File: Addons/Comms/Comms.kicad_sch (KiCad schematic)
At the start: 12 parts, among them J1 Conn_01x02, J2 Conn_02x06_Odd_Even, J3 Conn_01x02, J4 Conn_01x01, U1 SP3485EN

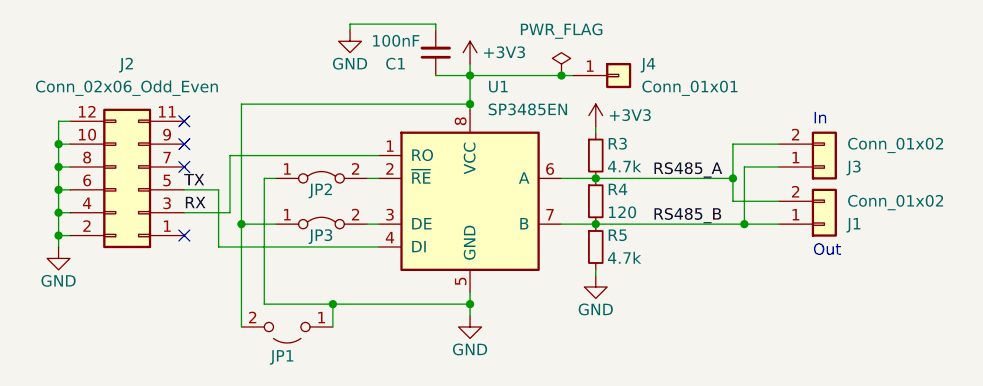
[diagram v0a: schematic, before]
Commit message: don't bridge 3v3 and ground lol
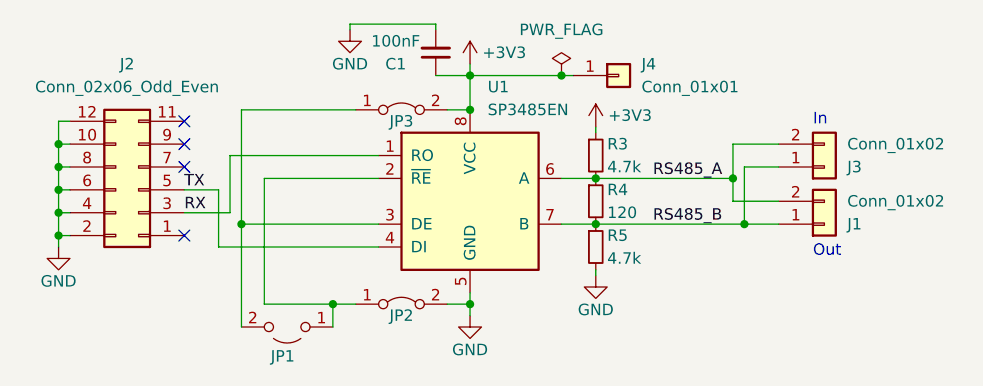
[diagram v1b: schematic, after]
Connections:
- net +3V3: now also JP3.2 (B); no longer JP1.2 (B), JP3.1 (A)
- net GND: now also JP2.2 (B); no longer JP1.1 (A), JP2.1 (A)
- net at U1.2 (~{RE}): now also JP1.1 (A), JP2.1 (A); no longer JP2.2 (B)
- net at U1.3 (DE): now also JP1.2 (B), JP3.1 (A); no longer JP3.2 (B)
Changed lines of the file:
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@@
   (junction (at 176.53 93.98) (diameter 0) (color 0 0 0 0)
   )
+  (junction (at 162.56 81.28) (diameter 0) (color 0 0 0 0)
+  )
   (junction (at 116.84 87.63) (diameter 0) (color 0 0 0 0)
   )
@@
   )
   (junction (at 116.84 90.17) (diameter 0) (color 0 0 0 0)
-  )
-  (junction (at 162.56 80.645) (diameter 0) (color 0 0 0 0)
   )
   (junction (at 116.84 92.71) (diameter 0) (color 0 0 0 0)
@@
     (stroke (width 0) (type default))
   )
-  (wire (pts (xy 147.32 102.87) (xy 162.56 102.87))
+  (wire (pts (xy 147.32 102.87) (xy 149.86 102.87))
     (stroke (width 0) (type default))
   )
@@
     (stroke (width 0) (type default))
   )
-  (wire (pts (xy 151.13 93.98) (xy 152.4 93.98))
-    (stroke (width 0) (type default))
-  )
   (wire (pts (xy 116.84 85.09) (xy 116.84 87.63))
     (stroke (width 0) (type default))
@@
     (stroke (width 0) (type default))
   )
+  (wire (pts (xy 160.02 102.87) (xy 162.56 102.87))
+    (stroke (width 0) (type default))
+  )
   (wire (pts (xy 130.81 90.17) (xy 134.62 90.17))
     (stroke (width 0) (type default))
@@
     (stroke (width 0) (type default))
   )
+  (wire (pts (xy 162.56 77.47) (xy 162.56 81.28))
+    (stroke (width 0) (type default))
+  )
   (wire (pts (xy 134.62 90.17) (xy 134.62 96.52))
     (stroke (width 0) (type default))
@@
     (stroke (width 0) (type default))
   )
-  (wire (pts (xy 140.97 88.9) (xy 139.7 88.9))
-    (stroke (width 0) (type default))
-  )
   (wire (pts (xy 149.225 71.755) (xy 158.75 71.755))
     (stroke (width 0) (type default))
@@
     (stroke (width 0) (type default))
   )
-  (wire (pts (xy 137.16 80.645) (xy 162.56 80.645))
+  (wire (pts (xy 137.16 81.28) (xy 149.86 81.28))
     (stroke (width 0) (type default))
   )
@@
     (stroke (width 0) (type default))
   )
-  (wire (pts (xy 137.16 93.98) (xy 137.16 80.645))
+  (wire (pts (xy 137.16 93.98) (xy 137.16 81.28))
     (stroke (width 0) (type default))
   )
@@
     (stroke (width 0) (type default))
   )
+  (wire (pts (xy 160.02 81.28) (xy 162.56 81.28))
+    (stroke (width 0) (type default))
+  )
   (wire (pts (xy 116.84 87.63) (xy 118.11 87.63))
     (stroke (width 0) (type default))
@@
     (stroke (width 0) (type default))
   )
-  (wire (pts (xy 152.4 88.9) (xy 151.13 88.9))
+  (wire (pts (xy 139.7 88.9) (xy 152.4 88.9))
     (stroke (width 0) (type default))
   )
@@
     (stroke (width 0) (type default))
   )
-  (wire (pts (xy 162.56 80.645) (xy 162.56 81.28))
-    (stroke (width 0) (type default))
-  )
   (wire (pts (xy 116.84 92.71) (xy 116.84 95.25))
     (stroke (width 0) (type default))
   )
-  (wire (pts (xy 137.16 93.98) (xy 140.97 93.98))
+  (wire (pts (xy 137.16 93.98) (xy 152.4 93.98))
     (stroke (width 0) (type default))
   )
   (wire (pts (xy 162.56 76.2) (xy 162.56 77.47))
-    (stroke (width 0) (type default))
-  )
-  (wire (pts (xy 162.56 77.47) (xy 162.56 80.645))
     (stroke (width 0) (type default))
   )
@@
         (path "/825aa7ba-79cf-4288-9f62-f278431e5a92"
           (reference "J1") (unit 1)
-        )
-      )
-    )
-  )
-  (symbol (lib_id "Jumper:Jumper_2_Bridged") (at 146.05 88.9 0) (unit 1)
-    (in_bom yes) (on_board yes) (dnp no)
-    (property "Reference" "JP2" (at 146.05 90.17 0)
-      (effects (font (size 1.27 1.27)))
-    )
-    (property "Value" "Jumper_2_Bridged" (at 146.05 86.36 0)
-      (effects (font (size 1.27 1.27)) hide)
-    )
-    (property "Footprint" "Jumper:SolderJumper-2_P1.3mm_Bridged_RoundedPad1.0x1.5mm" (at 146.05 88.9 0)
-      (effects (font (size 1.27 1.27)) hide)
-    )
-    (property "Datasheet" "~" (at 146.05 88.9 0)
-      (effects (font (size 1.27 1.27)) hide)
-    )
-    (pin "1")
-    (pin "2")
-    (instances
-      (project "Comms"
-        (path "/825aa7ba-79cf-4288-9f62-f278431e5a92"
-          (reference "JP2") (unit 1)
         )
       )
@@
     )
   )
-  (symbol (lib_id "Jumper:Jumper_2_Bridged") (at 146.05 93.98 0) (unit 1)
-    (in_bom yes) (on_board yes) (dnp no)
-    (property "Reference" "JP3" (at 146.05 95.25 0)
-      (effects (font (size 1.27 1.27)))
-    )
-    (property "Value" "Jumper_2_Bridged" (at 146.05 91.44 0)
-      (effects (font (size 1.27 1.27)) hide)
-    )
-    (property "Footprint" "Jumper:SolderJumper-2_P1.3mm_Bridged_RoundedPad1.0x1.5mm" (at 146.05 93.98 0)
-      (effects (font (size 1.27 1.27)) hide)
-    )
-    (property "Datasheet" "~" (at 146.05 93.98 0)
-      (effects (font (size 1.27 1.27)) hide)
-    )
-    (pin "1")
-    (pin "2")
-    (instances
-      (project "Comms"
-        (path "/825aa7ba-79cf-4288-9f62-f278431e5a92"
-          (reference "JP3") (unit 1)
-        )
-      )
-    )
-  )
   (symbol (lib_id "Connector_Generic:Conn_01x02") (at 201.93 87.63 0) (mirror x) (unit 1)
     (in_bom yes) (on_board yes) (dnp no)
@@
     )
   )
+  (symbol (lib_id "Jumper:Jumper_2_Bridged") (at 154.94 102.87 0) (unit 1)
+    (in_bom yes) (on_board yes) (dnp no)
+    (property "Reference" "JP2" (at 154.94 104.14 0)
+      (effects (font (size 1.27 1.27)))
+    )
+    (property "Value" "Jumper_2_Bridged" (at 154.94 100.33 0)
+      (effects (font (size 1.27 1.27)) hide)
+    )
+    (property "Footprint" "Jumper:SolderJumper-2_P1.3mm_Bridged_RoundedPad1.0x1.5mm" (at 154.94 102.87 0)
+      (effects (font (size 1.27 1.27)) hide)
+    )
+    (property "Datasheet" "~" (at 154.94 102.87 0)
+      (effects (font (size 1.27 1.27)) hide)
+    )
+    (pin "1")
+    (pin "2")
+    (instances
+      (project "Comms"
+        (path "/825aa7ba-79cf-4288-9f62-f278431e5a92"
+          (reference "JP2") (unit 1)
+        )
+      )
+    )
+  )
   (symbol (lib_id "power:GND") (at 176.53 99.695 0) (unit 1)
     (in_bom yes) (on_board yes) (dnp no)
@@
         )
       )
+    )
+  )
+  (symbol (lib_id "Jumper:Jumper_2_Bridged") (at 154.94 81.28 0) (unit 1)
+    (in_bom yes) (on_board yes) (dnp no)
+    (property "Reference" "JP3" (at 154.94 82.55 0)
+      (effects (font (size 1.27 1.27)))
+    )
+    (property "Value" "Jumper_2_Bridged" (at 154.94 78.74 0)
+      (effects (font (size 1.27 1.27)) hide)
+    )
+    (property "Footprint" "Jumper:SolderJumper-2_P1.3mm_Bridged_RoundedPad1.0x1.5mm" (at 154.94 81.28 0)
+      (effects (font (size 1.27 1.27)) hide)
+    )
+    (property "Datasheet" "~" (at 154.94 81.28 0)
+      (effects (font (size 1.27 1.27)) hide)
+    )
+    (pin "1")
+    (pin "2")
+    (instances
+      (project "Comms"
+        (path "/825aa7ba-79cf-4288-9f62-f278431e5a92"
+          (reference "JP3") (unit 1)
+        )
+      )

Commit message: Add RS485 functionality & addons, several fixes
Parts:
- C1: LCSC (none) -> C49678
- J1, J3: footprint Connector_PinHeader_2.54mm:PinHeader_1x02_P2.54mm_Horizontal -> Connector_JST:JST_XH_S2B-XH-A_1x02_P2.50mm_Horizontal
- R3, R5: LCSC (none) -> C17673
- R4: LCSC (none) -> C17437
- U1: LCSC (none) -> C8963
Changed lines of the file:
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@@
     (effects (font (size 1.27 1.27)) (justify left bottom))
-  )
-  (symbol (lib_id "Connector_Generic:Conn_01x02") (at 201.93 93.98 0) (mirror x) (unit 1)
-    (in_bom yes) (on_board yes) (dnp no)
-    (property "Reference" "J1" (at 204.47 93.98 0)
-      (effects (font (size 1.27 1.27)) (justify left))
-    )
-    (property "Value" "Conn_01x02" (at 204.47 91.44 0)
-      (effects (font (size 1.27 1.27)) (justify left))
-    )
-    (property "Footprint" "Connector_PinHeader_2.54mm:PinHeader_1x02_P2.54mm_Horizontal" (at 201.93 93.98 0)
-      (effects (font (size 1.27 1.27)) hide)
-    )
-    (property "Datasheet" "~" (at 201.93 93.98 0)
-      (effects (font (size 1.27 1.27)) hide)
-    )
-    (pin "1")
-    (pin "2")
-    (instances
-      (project "Comms"
-        (path "/825aa7ba-79cf-4288-9f62-f278431e5a92"
-          (reference "J1") (unit 1)
-        )
-      )
-    )
   )
   (symbol (lib_id "power:+3V3") (at 162.56 76.2 0) (unit 1)
@@
     )
     (property "Datasheet" "~" (at 125.73 90.17 0)
+      (effects (font (size 1.27 1.27)) hide)
+    )
+    (property "LCSC" "" (at 125.73 90.17 0)
       (effects (font (size 1.27 1.27)) hide)
     )
@@
       (effects (font (size 1.27 1.27)) hide)
     )
+    (property "LCSC" "C17673" (at 176.53 96.52 0)
+      (effects (font (size 1.27 1.27)) hide)
+    )
     (pin "1")
     (pin "2")
@@
       (effects (font (size 1.27 1.27)) hide)
     )
+    (property "LCSC" "C17673" (at 176.53 86.36 0)
+      (effects (font (size 1.27 1.27)) hide)
+    )
     (pin "1")
     (pin "2")
@@
     )
   )
+  (symbol (lib_id "Connector_Generic:Conn_01x02") (at 201.93 87.63 0) (mirror x) (unit 1)
+    (in_bom yes) (on_board yes) (dnp no)
+    (property "Reference" "J3" (at 204.47 87.63 0)
+      (effects (font (size 1.27 1.27)) (justify left))
+    )
+    (property "Value" "Conn_01x02" (at 204.47 85.09 0)
+      (effects (font (size 1.27 1.27)) (justify left))
+    )
+    (property "Footprint" "Connector_JST:JST_XH_S2B-XH-A_1x02_P2.50mm_Horizontal" (at 201.93 87.63 0)
+      (effects (font (size 1.27 1.27)) hide)
+    )
+    (property "Datasheet" "~" (at 201.93 87.63 0)
+      (effects (font (size 1.27 1.27)) hide)
+    )
+    (property "LCSC" "" (at 201.93 87.63 0)
+      (effects (font (size 1.27 1.27)) hide)
+    )
+    (pin "1")
+    (pin "2")
+    (instances
+      (project "Comms"
+        (path "/825aa7ba-79cf-4288-9f62-f278431e5a92"
+          (reference "J3") (unit 1)
+        )
+      )
+    )
+  )
   (symbol (lib_id "power:GND") (at 149.225 72.39 0) (unit 1)
     (in_bom yes) (on_board yes) (dnp no)
@@
       (effects (font (size 1.27 1.27)) hide)
     )
+    (property "LCSC" "C49678" (at 158.75 74.93 0)
+      (effects (font (size 1.27 1.27)) hide)
+    )
     (pin "1")
     (pin "2")
@@
     )
   )
-  (symbol (lib_id "Connector_Generic:Conn_01x02") (at 201.93 87.63 0) (mirror x) (unit 1)
-    (in_bom yes) (on_board yes) (dnp no)
-    (property "Reference" "J3" (at 204.47 87.63 0)
-      (effects (font (size 1.27 1.27)) (justify left))
-    )
-    (property "Value" "Conn_01x02" (at 204.47 85.09 0)
-      (effects (font (size 1.27 1.27)) (justify left))
-    )
-    (property "Footprint" "Connector_PinHeader_2.54mm:PinHeader_1x02_P2.54mm_Horizontal" (at 201.93 87.63 0)
-      (effects (font (size 1.27 1.27)) hide)
-    )
-    (property "Datasheet" "~" (at 201.93 87.63 0)
-      (effects (font (size 1.27 1.27)) hide)
-    )
-    (pin "1")
-    (pin "2")
-    (instances
-      (project "Comms"
-        (path "/825aa7ba-79cf-4288-9f62-f278431e5a92"
-          (reference "J3") (unit 1)
+  (symbol (lib_id "Connector_Generic:Conn_01x02") (at 201.93 93.98 0) (mirror x) (unit 1)
+    (in_bom yes) (on_board yes) (dnp no)
+    (property "Reference" "J1" (at 204.47 93.98 0)
+      (effects (font (size 1.27 1.27)) (justify left))
+    )
+    (property "Value" "Conn_01x02" (at 204.47 91.44 0)
+      (effects (font (size 1.27 1.27)) (justify left))
+    )
+    (property "Footprint" "Connector_JST:JST_XH_S2B-XH-A_1x02_P2.50mm_Horizontal" (at 201.93 93.98 0)
+      (effects (font (size 1.27 1.27)) hide)
+    )
+    (property "Datasheet" "~" (at 201.93 93.98 0)
+      (effects (font (size 1.27 1.27)) hide)
+    )
+    (property "LCSC" "" (at 201.93 93.98 0)
+      (effects (font (size 1.27 1.27)) hide)
+    )
+    (pin "1")
+    (pin "2")
+    (instances
+      (project "Comms"
+        (path "/825aa7ba-79cf-4288-9f62-f278431e5a92"
+          (reference "J1") (unit 1)
         )
       )
@@
       (effects (font (size 1.27 1.27)) hide)
     )
+    (property "LCSC" "" (at 179.07 77.47 0)
+      (effects (font (size 1.27 1.27)) hide)
+    )
     (pin "1")
     (instances
@@
     )
     (property "Datasheet" "http://www.icbase.com/pdf/SPX/SPX00480106.pdf" (at 162.56 91.44 0)
+      (effects (font (size 1.27 1.27)) hide)
+    )
+    (property "LCSC" " C8963" (at 162.56 91.44 0)
       (effects (font (size 1.27 1.27)) hide)
     )
@@
       (effects (font (size 1.27 1.27)) hide)
     )
+    (property "LCSC" "" (at 142.24 105.41 0)
+      (effects (font (size 1.27 1.27)) hide)
+    )
     (pin "1")
     (pin "2")
@@
       (effects (font (size 1.27 1.27)) hide)
     )
+    (property "LCSC" "C17437" (at 176.53 91.44 0)
+      (effects (font (size 1.27 1.27)) hide)
+    )
     (pin "1")
     (pin "2")
@@
       (effects (font (size 1.27 1.27)) hide)
     )
+    (property "LCSC" "" (at 154.94 102.87 0)
+      (effects (font (size 1.27 1.27)) hide)
+    )
     (pin "1")
     (pin "2")
@@
       (effects (font (size 1.27 1.27)) hide)
     )
+    (property "LCSC" "" (at 154.94 81.28 0)
+      (effects (font (size 1.27 1.27)) hide)
+    )
